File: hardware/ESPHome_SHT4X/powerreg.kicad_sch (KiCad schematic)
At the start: 15 parts, among them SW1 SW_Push, U2 BQ25628ERYKR

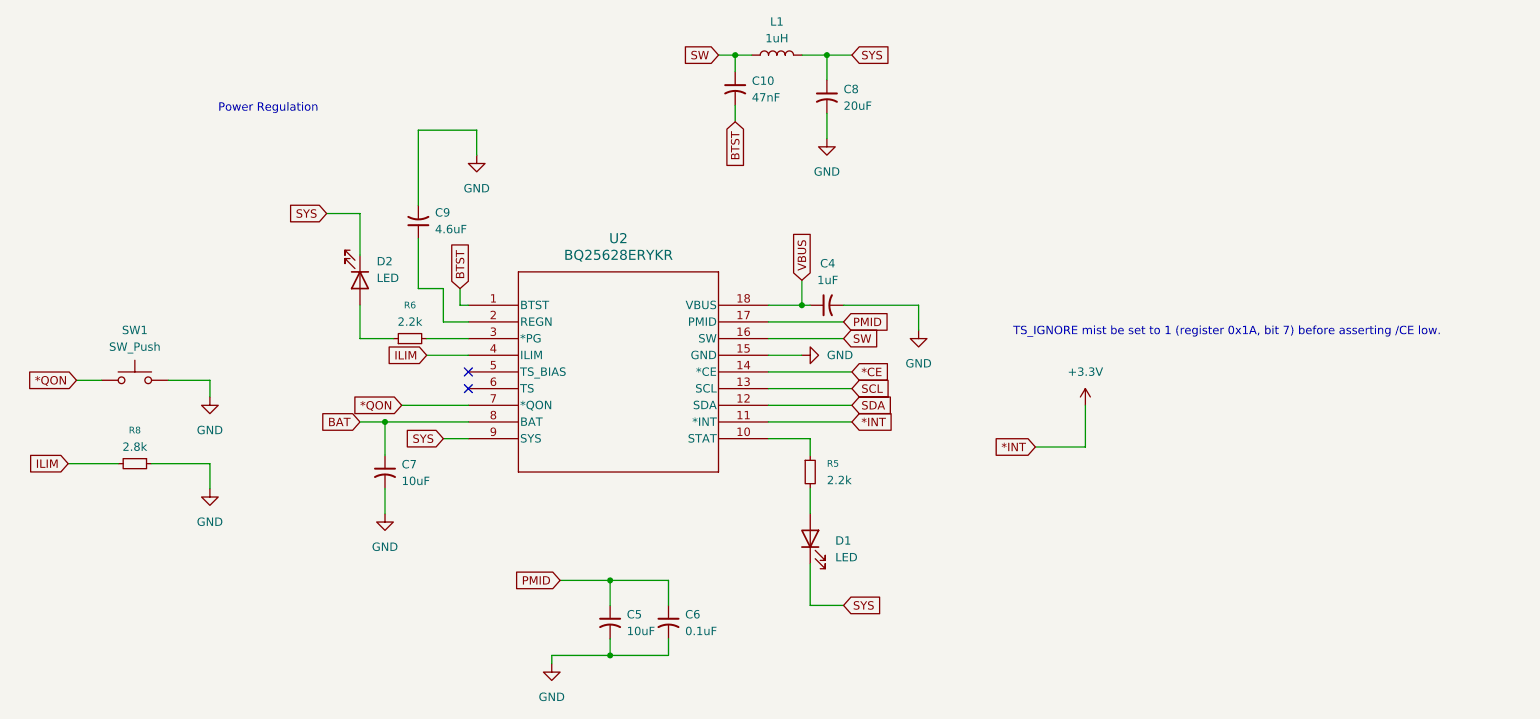
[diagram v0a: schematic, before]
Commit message: Finishing touches on schematic, started on PCB Design
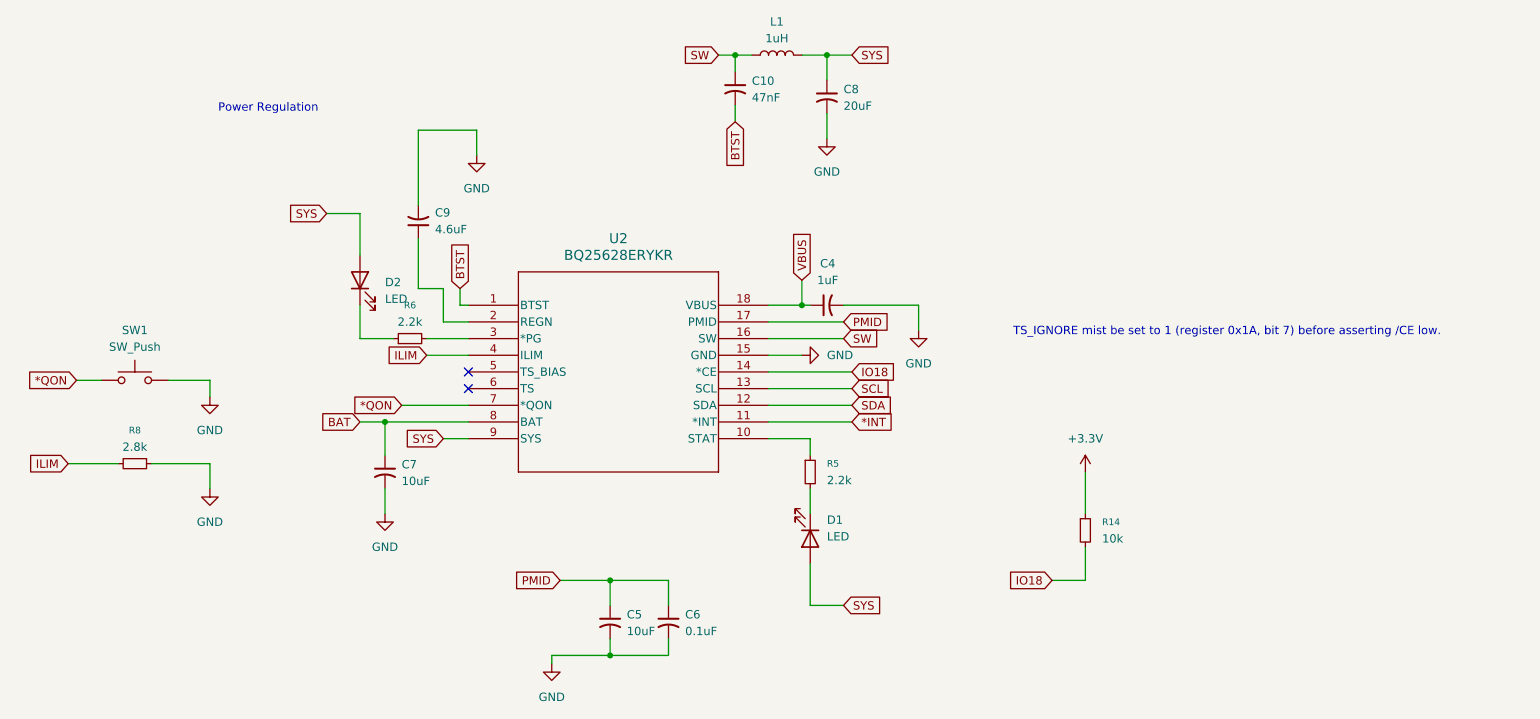
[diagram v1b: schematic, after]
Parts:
- added R14: 10k, Resistor_SMD:R_1206_3216Metric_Pad1.30x1.75mm_HandSolder, symbol Device:R_Small
- C10, C4, C5, C6, C7, C8, C9: footprint (none) -> Capacitor_SMD:C_1206_3216Metric_Pad1.33x1.80mm_HandSolder
- D1: footprint Package_DIP:DIP-8_W7.62mm -> LED_SMD:LED_1206_3216Metric_Pad1.42x1.75mm_HandSolder
- D2: footprint Button_Switch_THT:SW_NKK_GW12LJP -> LED_SMD:LED_1206_3216Metric_Pad1.42x1.75mm_HandSolder
- L1: footprint (none) -> Inductor_SMD:L_1206_3216Metric_Pad1.22x1.90mm_HandSolder
- R5, R6, R8: footprint Package_DIP:DIP-8_W7.62mm -> Resistor_SMD:R_1206_3216Metric_Pad1.30x1.75mm_HandSolder
- SW1: footprint (none) -> Library:SW_TS02-66-43-BK-100-SCR-D
- U2: footprint WQFN-HR18__RYK_TEX -> Library:WQFN-HR18__RYK_TEX
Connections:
- net +3.3V: now also R14.1; no longer U2.11 (*INT)
- net SYS: now also D1.2 (A), D2.2 (A); no longer D1.1 (K), D2.1 (K)
- net at R5.2: now also D1.1 (K); no longer D1.2 (A)
- net at R6.1: now also D2.1 (K); no longer D2.2 (A)
- net *CE renamed IO18
- net IO18: now also R14.2
- new net *INT: U2.11 (*INT)
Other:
- moved on the sheet: D1, D2

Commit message: Making progress
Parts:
- C10, C4, C5, C6, C7, C8, C9: footprint Capacitor_SMD:C_1206_3216Metric_Pad1.33x1.80mm_HandSolder -> Capacitor_SMD:C_01005_0402Metric_Pad0.57x0.30mm_HandSolder
- L1: footprint Inductor_SMD:L_1206_3216Metric_Pad1.22x1.90mm_HandSolder -> Resistor_SMD:R_01005_0402Metric_Pad0.57x0.30mm_HandSolder
- R14, R5, R6: footprint Resistor_SMD:R_1206_3216Metric_Pad1.30x1.75mm_HandSolder -> Resistor_SMD:R_01005_0402Metric_Pad0.57x0.30mm_HandSolder
- R8: footprint Resistor_SMD:R_1206_3216Metric_Pad1.30x1.75mm_HandSolder -> Inductor_SMD:L_01005_0402Metric_Pad0.57x0.30mm_HandSolder
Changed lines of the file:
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@@
 			)
 		)
-		(property "Footprint" "Inductor_SMD:L_1206_3216Metric_Pad1.22x1.90mm_HandSolder"
+		(property "Footprint" "Resistor_SMD:R_01005_0402Metric_Pad0.57x0.30mm_HandSolder"
 			(at 156.21 39.37 0)
 			(hide yes)
@@
 			)
 		)
-		(property "Footprint" "Capacitor_SMD:C_1206_3216Metric_Pad1.33x1.80mm_HandSolder"
+		(property "Footprint" "Capacitor_SMD:C_01005_0402Metric_Pad0.57x0.30mm_HandSolder"
 			(at 130.81 125.73 0)
 			(hide yes)
@@
 			)
 		)
-		(property "Footprint" "Resistor_SMD:R_1206_3216Metric_Pad1.30x1.75mm_HandSolder"
+		(property "Footprint" "Resistor_SMD:R_01005_0402Metric_Pad0.57x0.30mm_HandSolder"
 			(at 161.29 102.87 0)
 			(hide yes)
@@
 			)
 		)
-		(property "Footprint" "Resistor_SMD:R_1206_3216Metric_Pad1.30x1.75mm_HandSolder"
+		(property "Footprint" "Inductor_SMD:L_01005_0402Metric_Pad0.57x0.30mm_HandSolder"
 			(at 58.42 101.6 0)
 			(hide yes)
@@
 			)
 		)
-		(property "Footprint" "Resistor_SMD:R_1206_3216Metric_Pad1.30x1.75mm_HandSolder"
+		(property "Footprint" "Resistor_SMD:R_01005_0402Metric_Pad0.57x0.30mm_HandSolder"
 			(at 203.2 111.76 0)
 			(hide yes)
@@
 			)
 		)
-		(property "Footprint" "Capacitor_SMD:C_1206_3216Metric_Pad1.33x1.80mm_HandSolder"
+		(property "Footprint" "Capacitor_SMD:C_01005_0402Metric_Pad0.57x0.30mm_HandSolder"
 			(at 139.7 125.73 0)
 			(hide yes)
@@
 			)
 		)
-		(property "Footprint" "Capacitor_SMD:C_1206_3216Metric_Pad1.33x1.80mm_HandSolder"
+		(property "Footprint" "Capacitor_SMD:C_01005_0402Metric_Pad0.57x0.30mm_HandSolder"
 			(at 149.86 44.45 0)
 			(hide yes)
@@
 			)
 		)
-		(property "Footprint" "Capacitor_SMD:C_1206_3216Metric_Pad1.33x1.80mm_HandSolder"
+		(property "Footprint" "Capacitor_SMD:C_01005_0402Metric_Pad0.57x0.30mm_HandSolder"
 			(at 96.52 102.87 0)
 			(hide yes)
@@
 			)
 		)
-		(property "Footprint" "Resistor_SMD:R_1206_3216Metric_Pad1.30x1.75mm_HandSolder"
+		(property "Footprint" "Resistor_SMD:R_01005_0402Metric_Pad0.57x0.30mm_HandSolder"
 			(at 100.33 82.55 0)
 			(hide yes)
@@
 			)
 		)
-		(property "Footprint" "Capacitor_SMD:C_1206_3216Metric_Pad1.33x1.80mm_HandSolder"
+		(property "Footprint" "Capacitor_SMD:C_01005_0402Metric_Pad0.57x0.30mm_HandSolder"
 			(at 101.6 64.77 0)
 			(hide yes)
@@
 			)
 		)
-		(property "Footprint" "Capacitor_SMD:C_1206_3216Metric_Pad1.33x1.80mm_HandSolder"
+		(property "Footprint" "Capacitor_SMD:C_01005_0402Metric_Pad0.57x0.30mm_HandSolder"
 			(at 163.83 45.72 0)
 			(hide yes)
@@
 			)
 		)
-		(property "Footprint" "Capacitor_SMD:C_1206_3216Metric_Pad1.33x1.80mm_HandSolder"
+		(property "Footprint" "Capacitor_SMD:C_01005_0402Metric_Pad0.57x0.30mm_HandSolder"
 			(at 163.83 77.47 0)
 			(hide yes)
@@
 		)
 	)
+	(embedded_fonts no)
 )

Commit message: making progress
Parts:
- C10, C4, C5, C6, C7, C8, C9: footprint Capacitor_SMD:C_01005_0402Metric_Pad0.57x0.30mm_HandSolder -> Capacitor_SMD:C_0201_0603Metric_Pad0.64x0.40mm_HandSolder
- L1, R14, R5, R6: footprint Resistor_SMD:R_01005_0402Metric_Pad0.57x0.30mm_HandSolder -> Resistor_SMD:R_0201_0603Metric_Pad0.64x0.40mm_HandSolder
- R8: footprint Inductor_SMD:L_01005_0402Metric_Pad0.57x0.30mm_HandSolder -> Inductor_SMD:L_0201_0603Metric_Pad0.64x0.40mm_HandSolder
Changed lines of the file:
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@@
 			)
 		)
-		(property "Footprint" "Resistor_SMD:R_01005_0402Metric_Pad0.57x0.30mm_HandSolder"
+		(property "Footprint" "Resistor_SMD:R_0201_0603Metric_Pad0.64x0.40mm_HandSolder"
 			(at 156.21 39.37 0)
 			(hide yes)
@@
 			)
 		)
-		(property "Footprint" "Capacitor_SMD:C_01005_0402Metric_Pad0.57x0.30mm_HandSolder"
+		(property "Footprint" "Capacitor_SMD:C_0201_0603Metric_Pad0.64x0.40mm_HandSolder"
 			(at 130.81 125.73 0)
 			(hide yes)
@@
 			)
 		)
-		(property "Footprint" "Resistor_SMD:R_01005_0402Metric_Pad0.57x0.30mm_HandSolder"
+		(property "Footprint" "Resistor_SMD:R_0201_0603Metric_Pad0.64x0.40mm_HandSolder"
 			(at 161.29 102.87 0)
 			(hide yes)
@@
 			)
 		)
-		(property "Footprint" "Inductor_SMD:L_01005_0402Metric_Pad0.57x0.30mm_HandSolder"
+		(property "Footprint" "Inductor_SMD:L_0201_0603Metric_Pad0.64x0.40mm_HandSolder"
 			(at 58.42 101.6 0)
 			(hide yes)
@@
 			)
 		)
-		(property "Footprint" "Resistor_SMD:R_01005_0402Metric_Pad0.57x0.30mm_HandSolder"
+		(property "Footprint" "Resistor_SMD:R_0201_0603Metric_Pad0.64x0.40mm_HandSolder"
 			(at 203.2 111.76 0)
 			(hide yes)
@@
 			)
 		)
-		(property "Footprint" "Capacitor_SMD:C_01005_0402Metric_Pad0.57x0.30mm_HandSolder"
+		(property "Footprint" "Capacitor_SMD:C_0201_0603Metric_Pad0.64x0.40mm_HandSolder"
 			(at 139.7 125.73 0)
 			(hide yes)
@@
 			)
 		)
-		(property "Footprint" "Capacitor_SMD:C_01005_0402Metric_Pad0.57x0.30mm_HandSolder"
+		(property "Footprint" "Capacitor_SMD:C_0201_0603Metric_Pad0.64x0.40mm_HandSolder"
 			(at 149.86 44.45 0)
 			(hide yes)
@@
 			)
 		)
-		(property "Footprint" "Capacitor_SMD:C_01005_0402Metric_Pad0.57x0.30mm_HandSolder"
+		(property "Footprint" "Capacitor_SMD:C_0201_0603Metric_Pad0.64x0.40mm_HandSolder"
 			(at 96.52 102.87 0)
 			(hide yes)
@@
 			)
 		)
-		(property "Footprint" "Resistor_SMD:R_01005_0402Metric_Pad0.57x0.30mm_HandSolder"
+		(property "Footprint" "Resistor_SMD:R_0201_0603Metric_Pad0.64x0.40mm_HandSolder"
 			(at 100.33 82.55 0)
 			(hide yes)
@@
 			)
 		)
-		(property "Footprint" "Capacitor_SMD:C_01005_0402Metric_Pad0.57x0.30mm_HandSolder"
+		(property "Footprint" "Capacitor_SMD:C_0201_0603Metric_Pad0.64x0.40mm_HandSolder"
 			(at 101.6 64.77 0)
 			(hide yes)
@@
 			)
 		)
-		(property "Footprint" "Capacitor_SMD:C_01005_0402Metric_Pad0.57x0.30mm_HandSolder"
+		(property "Footprint" "Capacitor_SMD:C_0201_0603Metric_Pad0.64x0.40mm_HandSolder"
 			(at 163.83 45.72 0)
 			(hide yes)
@@
 			)
 		)
-		(property "Footprint" "Capacitor_SMD:C_01005_0402Metric_Pad0.57x0.30mm_HandSolder"
+		(property "Footprint" "Capacitor_SMD:C_0201_0603Metric_Pad0.64x0.40mm_HandSolder"
 			(at 163.83 77.47 0)
 			(hide yes)
@@
 		)
 	)
-	(embedded_fonts no)
 )

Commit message: making more progress
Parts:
- U2: footprint Library:WQFN-HR18__RYK_TEX -> ESPhome:WQFN-HR18__RYK_TEX
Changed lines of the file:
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@@
 			)
 		)
-		(property "Footprint" "Library:WQFN-HR18__RYK_TEX"
+		(property "Footprint" "ESPhome:WQFN-HR18__RYK_TEX"
 			(at 109.22 77.47 0)
 			(hide yes)
